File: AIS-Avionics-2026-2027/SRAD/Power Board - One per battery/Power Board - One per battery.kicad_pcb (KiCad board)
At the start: 2 copper layers, 112.5 x 37.5 mm, 3 parts, among them J1 Conn_01x02, J2 Conn_01x02

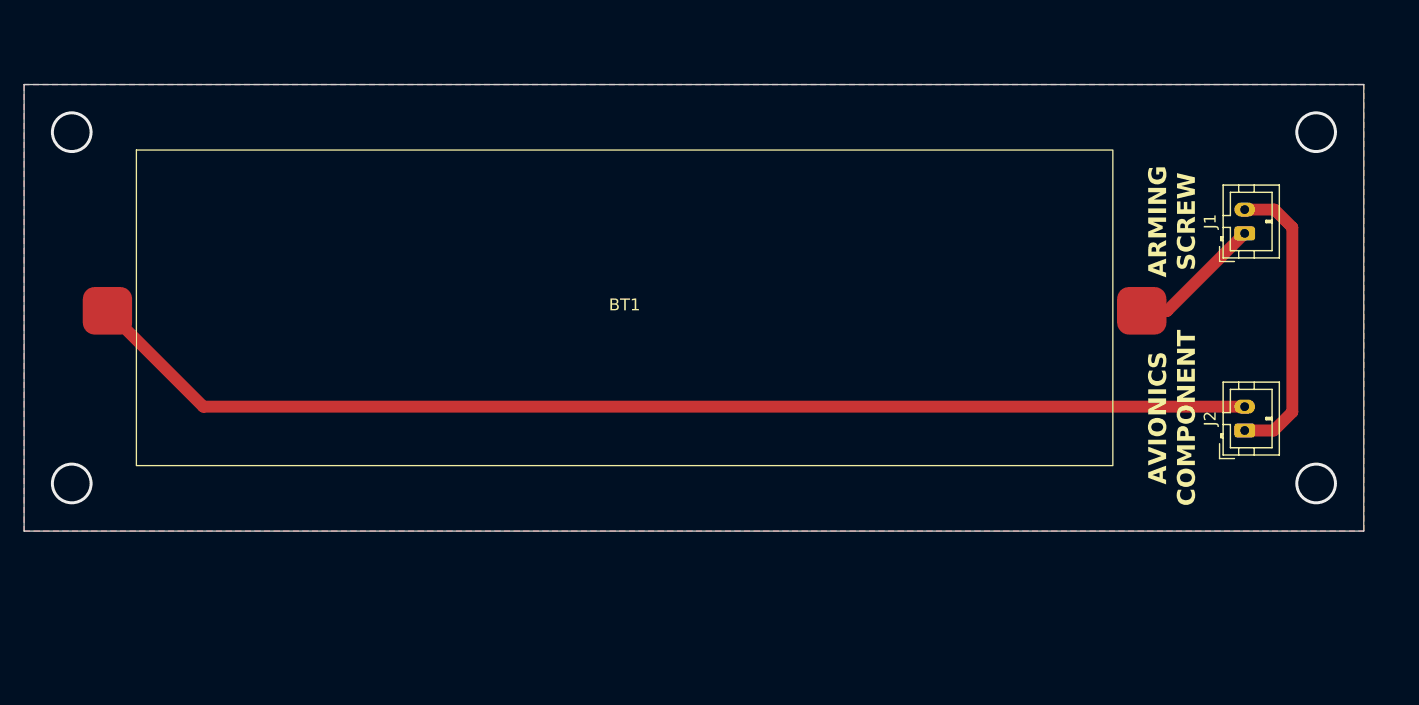
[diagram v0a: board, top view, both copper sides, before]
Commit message: Battery shenanigans.
So many battery shenanigans
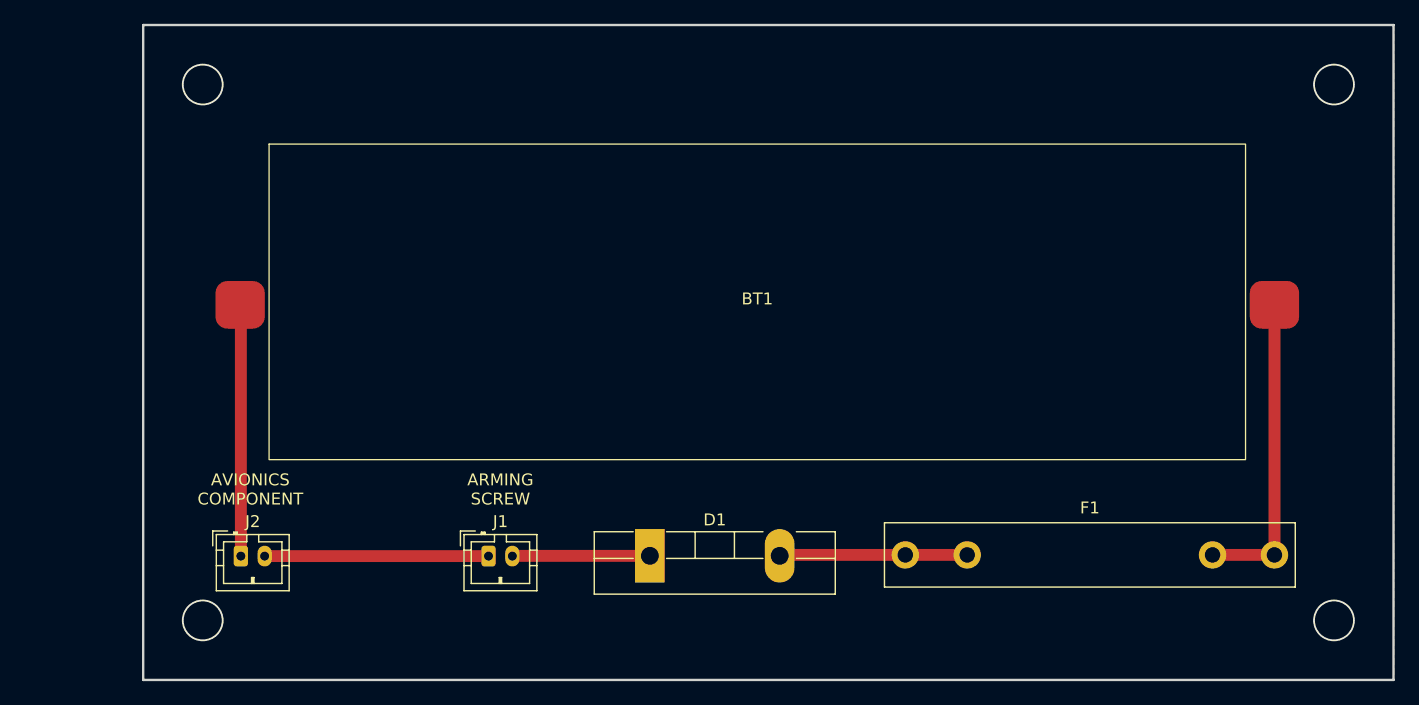
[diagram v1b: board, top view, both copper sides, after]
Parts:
- added D1: D, Package_TO_SOT_THT:TO-264-2_Vertical, F.Cu at (137.6, 84.6)
- added F1: Fuse, Fuse:Fuseholder_Littelfuse_445_030_series_5x30mm, F.Cu at (159.0, 84.5)
- J1, J2: value Conn_01x02 -> Conn_01x02_Pin; footprint Reconfigured Standard Components:JST_PH_B2B-PH-K_1x02_P2.00mm_Vertical_CAD_Fixed -> Connector_JST:JST_PH_B2B-PH-K_1x02_P2.00mm_Vertical
- moved J2 85.0 mm to (103.2, 84.6), turned to 0 degrees
- moved J1 69.0 mm to (124.0, 84.6), turned to 0 degrees
- moved BT1 11.2 mm to (146.6, 63.5)
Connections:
- J1 pad 1: Net-(BT1-+) -> Net-(J1-Pin_1)
- J1 pad 2: Net-(J1-Pin_2) -> Net-(D1-K)
- J2 pad 1: Net-(J1-Pin_2) -> Net-(BT1--)
- J2 pad 2: Net-(BT1--) -> Net-(J1-Pin_1)
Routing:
- net Net-(BT1--): track 98.8 -> 21.1 mm
- net Net-(J1-Pin_2): track 24.8 -> 0.00 mm
- net Net-(J1-Pin_1): track 0.00 -> 18.8 mm
- net Net-(D1-A): track 0.00 -> 15.8 mm
- net Net-(BT1-+): track 11.3 -> 26.2 mm
- net Net-(D1-K): track 0.00 -> 11.6 mm
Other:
- board size 112.5 x 37.5 mm -> 105 x 55 mm
